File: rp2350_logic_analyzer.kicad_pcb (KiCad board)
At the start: 4 copper layers, 65.1 x 34 mm, 35 parts, among them J1 Conn_02x04, J2 Conn_01x03, J3 Conn_01x03, J4 Conn_01x03, J5 Conn_01x03, U2 TLV3501AIDBV, U3 TLV3501AIDBV, U4 TLV3501AIDBV, U5 TLV3501AIDBV, U6 SRV05-4, U7 Si8661BD-B-IS

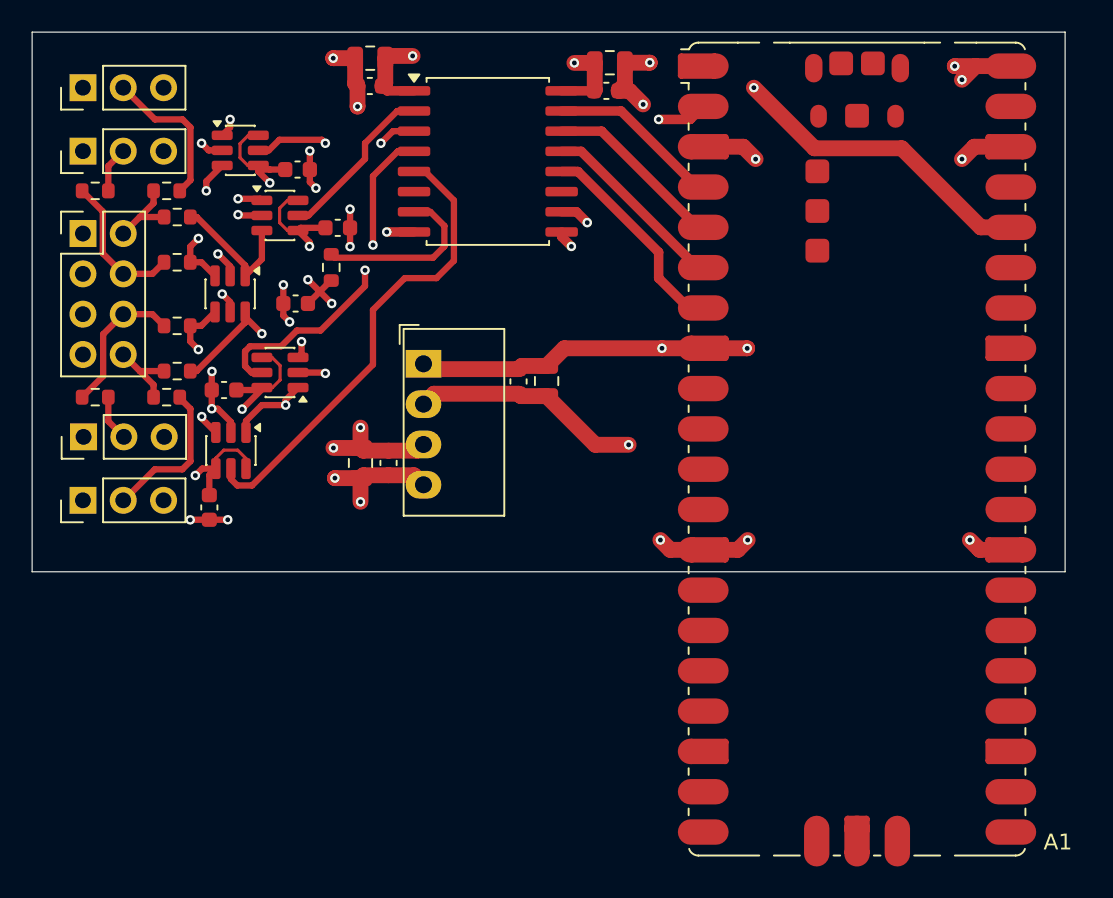
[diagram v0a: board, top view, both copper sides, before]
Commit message: Improve grounding
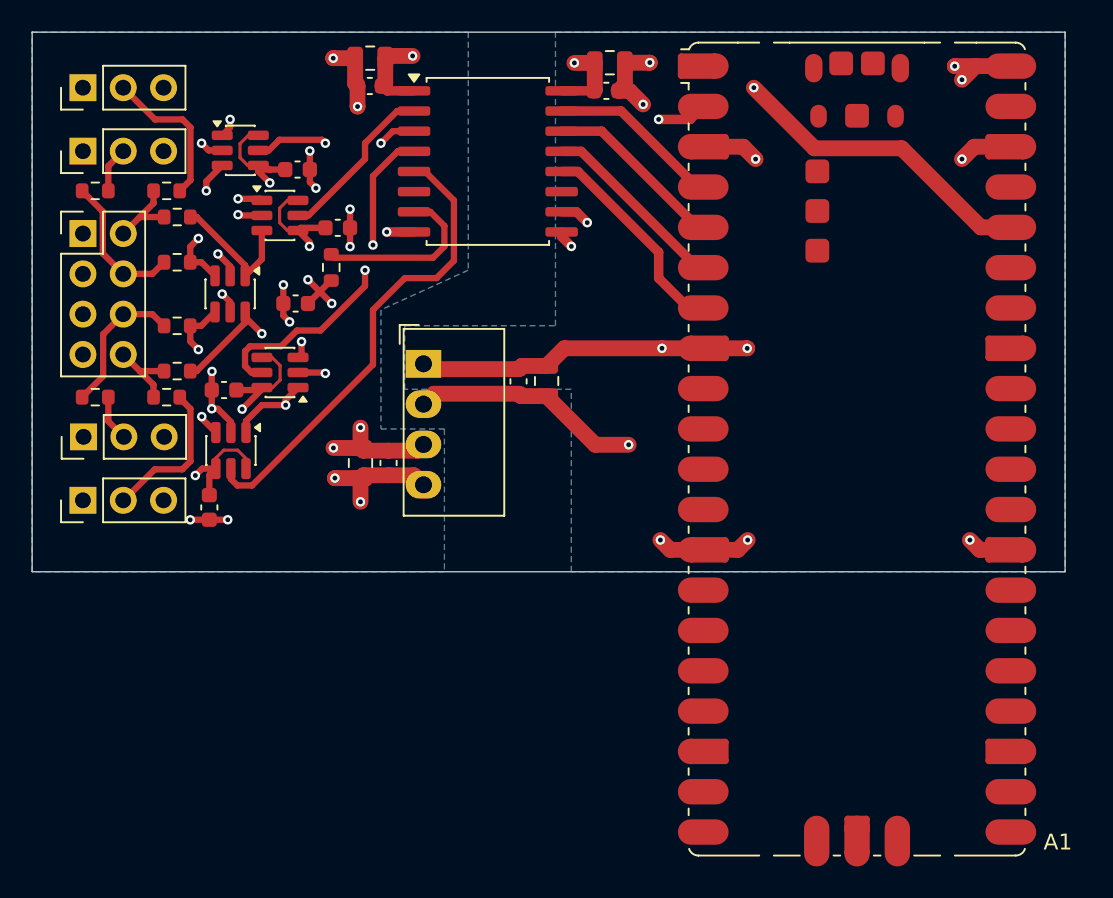
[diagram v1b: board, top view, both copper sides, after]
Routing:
- added copper zone on B.Cu, net /GND
- added copper zone on B.Cu, net /GND_ISO
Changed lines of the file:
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@@
 			(pinfunction "Pin_1")
 			(pintype "passive")
+			(zone_connect 2)
 		)
 		(pad "2" thru_hole circle
@@
 			(pinfunction "Pin_1")
 			(pintype "passive")
+			(zone_connect 2)
 		)
 		(pad "2" thru_hole circle
@@
 			(pinfunction "Pin_1")
 			(pintype "passive")
+			(zone_connect 2)
 		)
 		(pad "2" thru_hole circle
@@
 			(pinfunction "Pin_1")
 			(pintype "passive")
+			(zone_connect 2)
 		)
 		(pad "2" thru_hole circle
@@
 			(pinfunction "Pin_3")
 			(pintype "passive")
+			(zone_connect 2)
 		)
 		(pad "4" thru_hole circle
@@
 			(pinfunction "Pin_5")
 			(pintype "passive")
+			(zone_connect 2)
 		)
 		(pad "6" thru_hole circle
@@
 			(pinfunction "Pin_7")
 			(pintype "passive")
+			(zone_connect 2)
 		)
 		(pad "8" thru_hole circle
@@
 			(pinfunction "Pin_1")
 			(pintype "passive")
+			(zone_connect 2)
 		)
 		(pad "2" thru_hole circle
@@
 			(pinfunction "-Vin")
 			(pintype "power_in")
+			(zone_connect 2)
 		)
 		(pad "2" thru_hole oval
@@
 			(pinfunction "-Vout")
 			(pintype "power_out")
+			(zone_connect 2)
 		)
 		(pad "4" thru_hole oval
@@
 		(net 9)
 		(net_name "/GND")
+		(layer "B.Cu")
+		(hatch edge 0.5)
+		(priority 3)
+		(connect_pads
+			(clearance 0.25)
+		)
+		(min_thickness 0.25)
+		(filled_areas_thickness no)
+		(fill yes
+			(thermal_gap 0.5)
+			(thermal_bridge_width 0.4)
+		)
+		(polygon
+			(pts
+				(xy 51.5 17) (xy 83.614524 16.999999) (xy 83.608129 51) (xy 52.5 51) (xy 52.5 39.5) (xy 42 39.5)
+				(xy 42 35.5) (xy 51.5 35.5)
+			)
+		)
+	)
+	(zone
+		(net 44)
+		(net_name "/GND_ISO")
+		(layer "B.Cu")
+		(hatch edge 0.5)
+		(priority 2)
+		(connect_pads
+			(clearance 0.25)
+		)
+		(min_thickness 0.25)
+		(filled_areas_thickness no)
+		(fill yes
+			(thermal_gap 0.5)
+			(thermal_bridge_width 0.4)
+		)
+		(polygon
+			(pts
+				(xy 18.5 17) (xy 46 17) (xy 46 32) (xy 40.5 34.5) (xy 40.5 42) (xy 44.5 42) (xy 44.5 51) (xy 18.5 51)
+			)
+		)
+	)
+	(zone
+		(net 9)
+		(net_name "/GND")
 		(layer "In1.Cu")
 		(hatch edge 0.5)
 		(priority 1)
 		(connect_pads
-			(clearance 0.5)
+			(clearance 0.25)
 		)
-		(min_thickness 1)
+		(min_thickness 0.25)
 		(filled_areas_thickness no)
 		(fill yes
 			(thermal_gap 0.5)
-			(thermal_bridge_width 1)
+			(thermal_bridge_width 0.4)
 		)
 		(polygon
 			(pts
-				(xy 83.61 17) (xy 51.61 17) (xy 51.61 35.5) (xy 42.11 35.5) (xy 42.11 39.5) (xy 52.61 39.5) (xy 52.61 51)
+				(xy 83.61 17) (xy 51.5 17) (xy 51.5 35.5) (xy 42 35.5) (xy 42 39.5) (xy 52.5 39.5) (xy 52.5 51)
 				(xy 83.61 51)
 			)
@@
 		(hatch edge 0.5)
 		(connect_pads
-			(clearance 0.5)
+			(clearance 0.25)
 		)
-		(min_thickness 1)
+		(min_thickness 0.25)
 		(filled_areas_thickness no)
 		(fill yes
 			(thermal_gap 0.5)
-			(thermal_bridge_width 1)
+			(thermal_bridge_width 0.4)
 		)
 		(polygon
